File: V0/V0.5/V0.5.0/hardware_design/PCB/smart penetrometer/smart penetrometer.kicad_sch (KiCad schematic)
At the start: 28 parts, among them J1 Conn_01x02_Female, J2 XLR3_Switched, J3 Conn_01x07_Female, J4 Screw_Terminal, J5 Conn_02x04, U1 ADS1120IRVAR, U2 DS3231M, U3 BME260, U4 ADS1115IRUGT, U5 VO615A

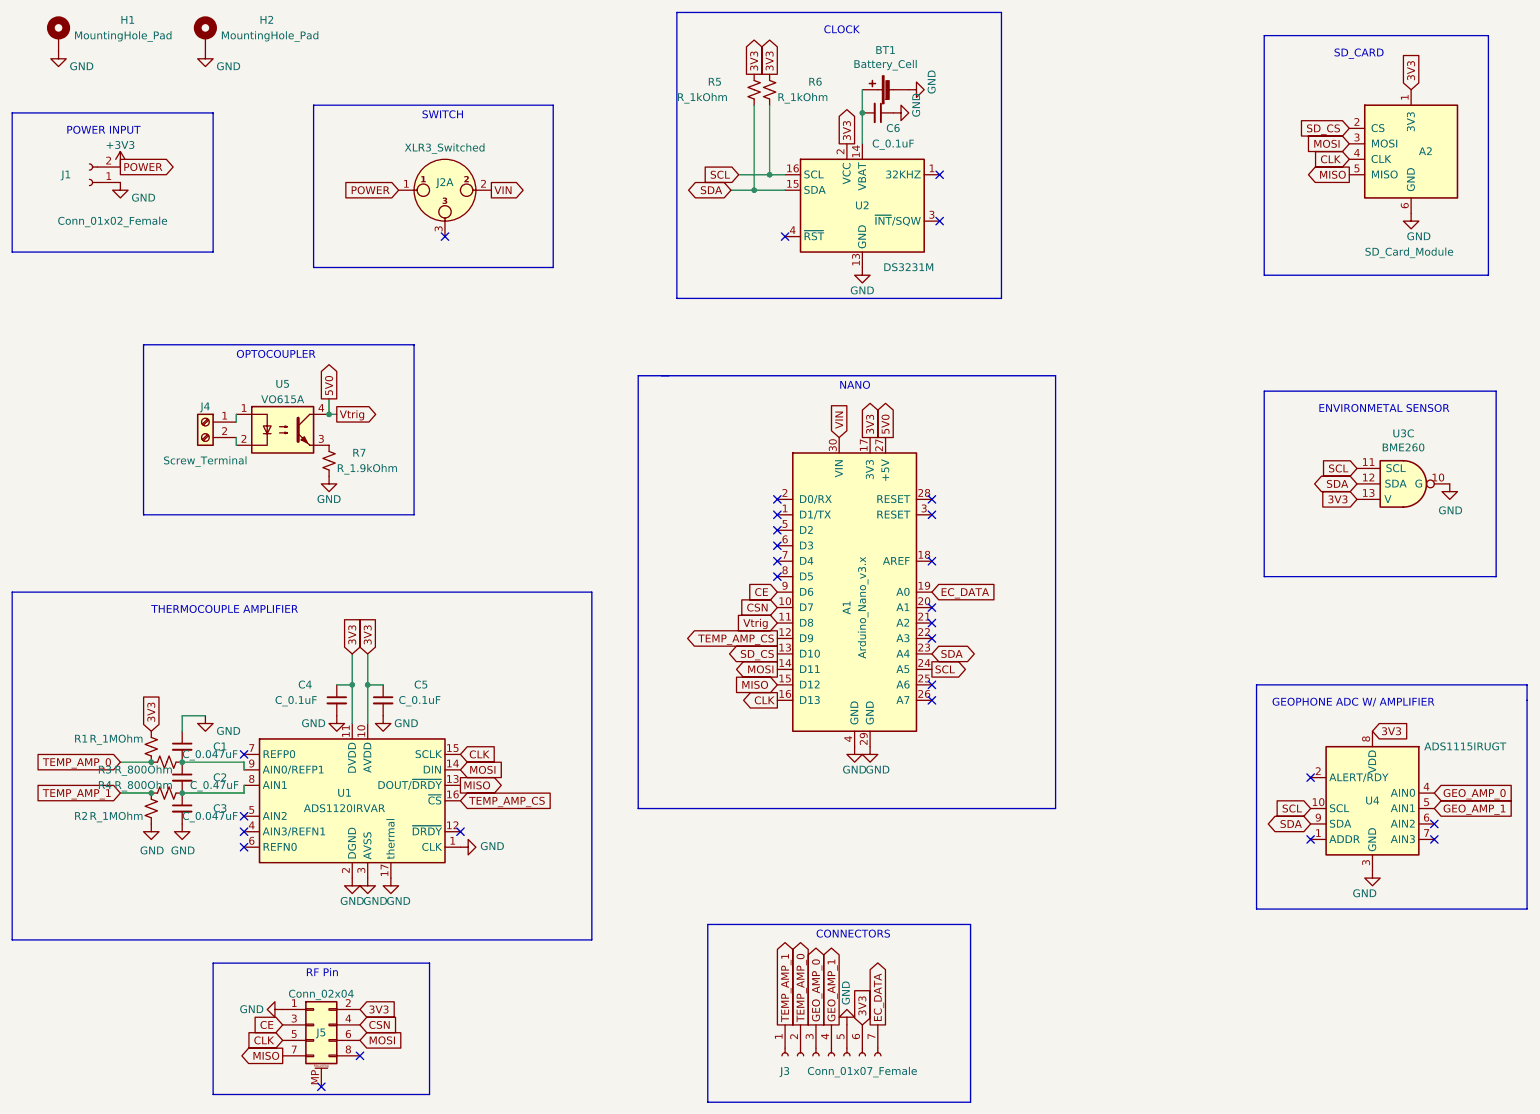
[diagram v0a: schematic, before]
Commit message: PCB update
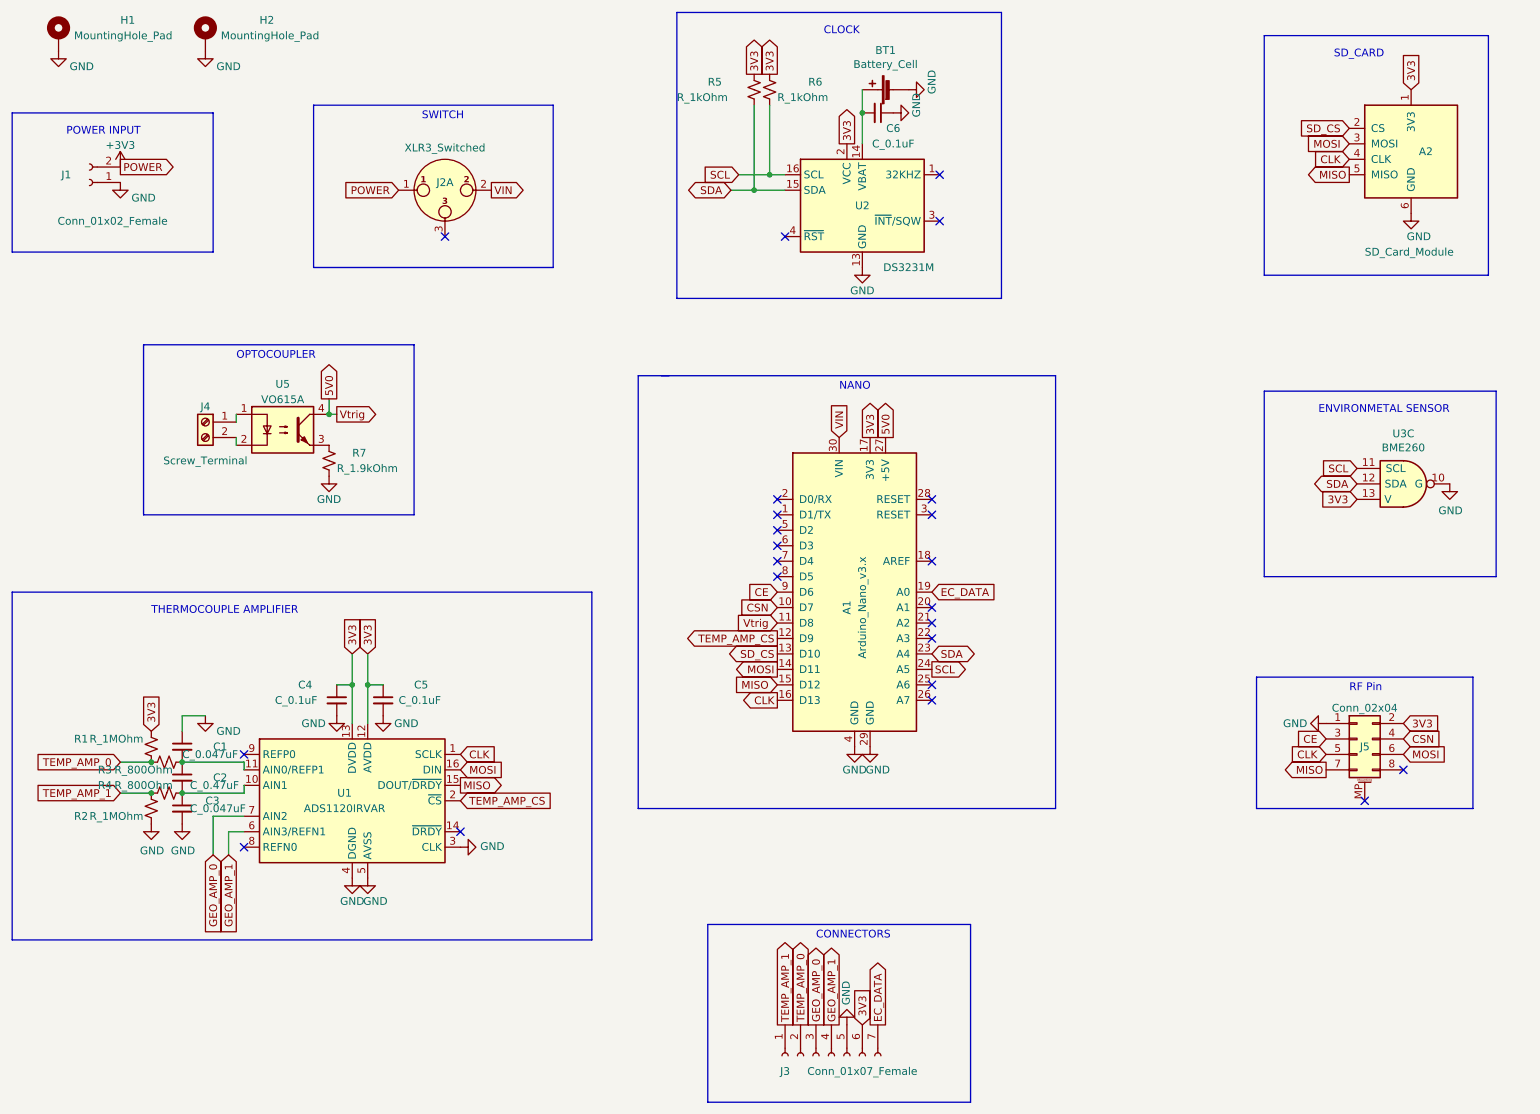
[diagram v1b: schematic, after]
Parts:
- removed U4: ADS1115IRUGT, kitest:10X2QFN, symbol Analog_ADC:ADS1115IDGS
- U1: footprint Package_DFN_QFN:VQFN-16-1EP_3x3mm_P0.5mm_EP1.45x1.45mm_ThermalVias -> kitest:ADS1120IPW 16TSSOP
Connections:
- net 3V3: now also U1.12 (AVDD), U1.13 (DVDD); no longer U1.10 (AVDD), U1.11 (DVDD)
- net CLK: now also U1.1 (SCLK); no longer U1.15 (SCLK)
- net GEO_AMP_0: now also U1.7 (AIN2)
- net GEO_AMP_1: now also U1.6 (AIN3/REFN1)
- net GND: now also U1.4 (DGND), U1.5 (AVSS); no longer U1.1 (CLK), U1.17 (thermal), U1.2 (DGND)
- net MISO: now also U1.15 (DOUT/~{DRDY}); no longer U1.13 (DOUT/~{DRDY})
- net MOSI: now also U1.16 (DIN); no longer U1.14 (DIN)
- net TEMP_AMP_CS: now also U1.2 (~{CS}); no longer U1.16 (~{CS})
- net at C1.2, C2.1, R3.1: now also U1.11 (AIN0/REFP1); no longer U1.9 (AIN0/REFP1)
- net at C2.2, C3.1, R4.1: now also U1.10 (AIN1); no longer U1.8 (AIN1)
- no-connect marks 29 -> 23
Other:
- note removed: "GEOPHONE ADC W/ AMPLIFIER"
- moved on the sheet: J5
